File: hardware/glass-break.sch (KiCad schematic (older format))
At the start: 33 parts, among them P1 USB_OTG, SW1 SW_PUSH, SW2 SW_PUSH, SW3 SW_PUSH, U1 ESP-WROOM-02, U11 SPX3819, U2 OP275, U3 electret_microphone

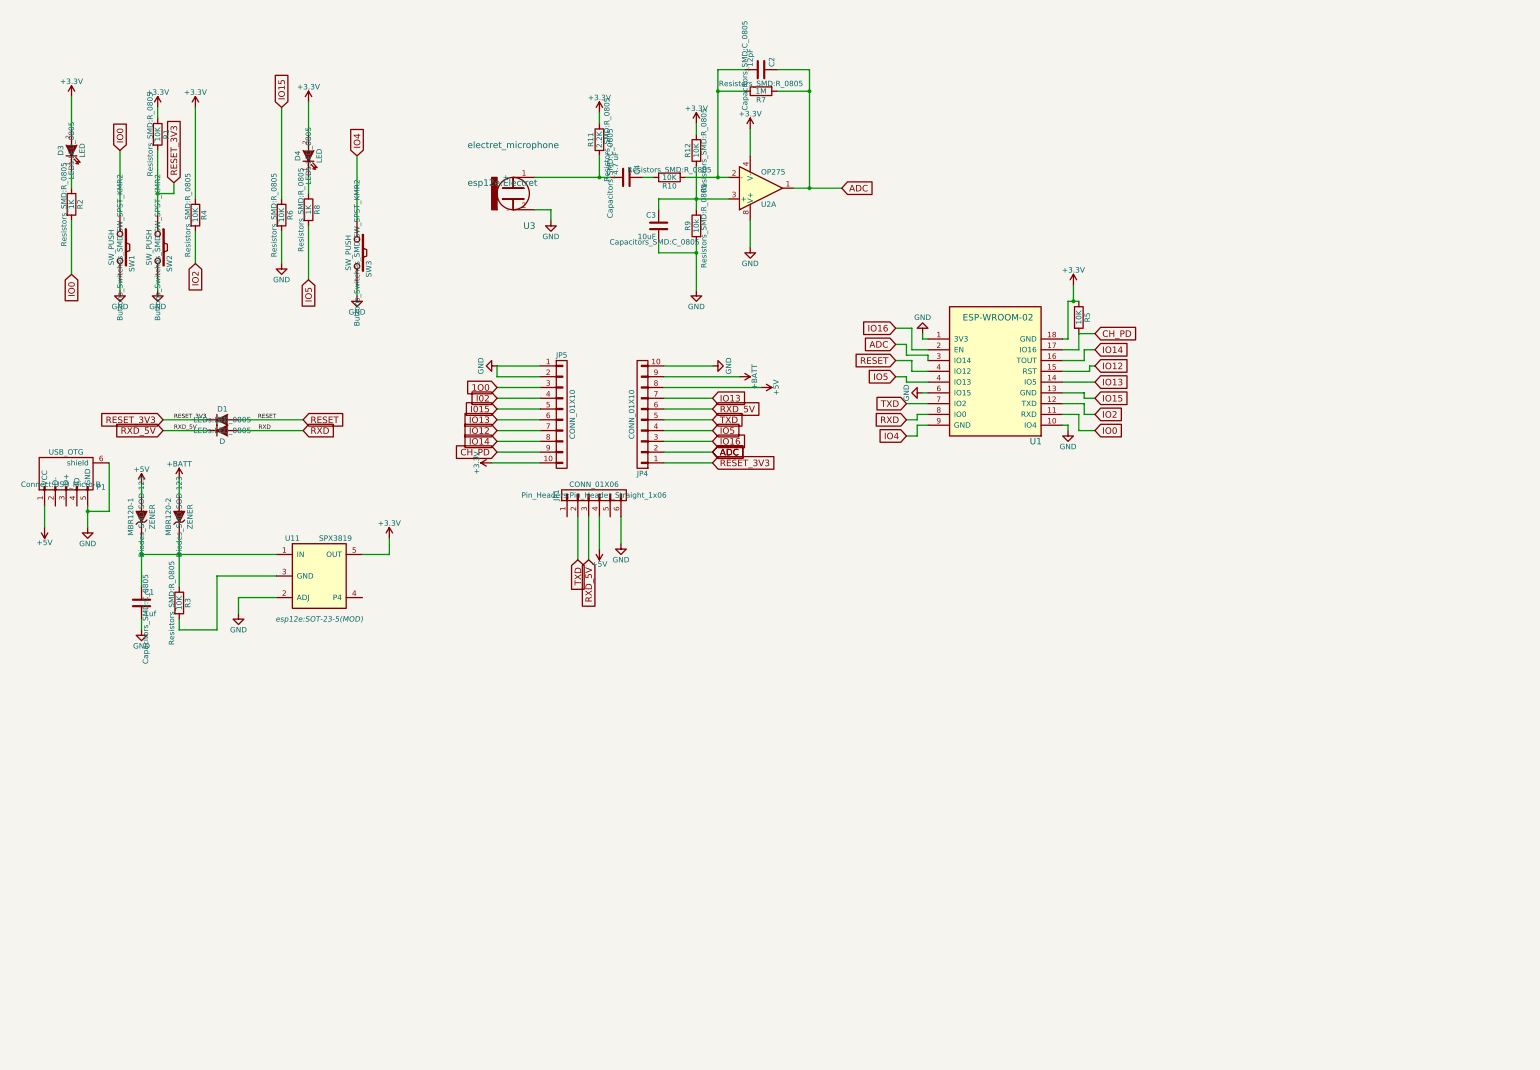
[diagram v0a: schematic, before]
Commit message: update
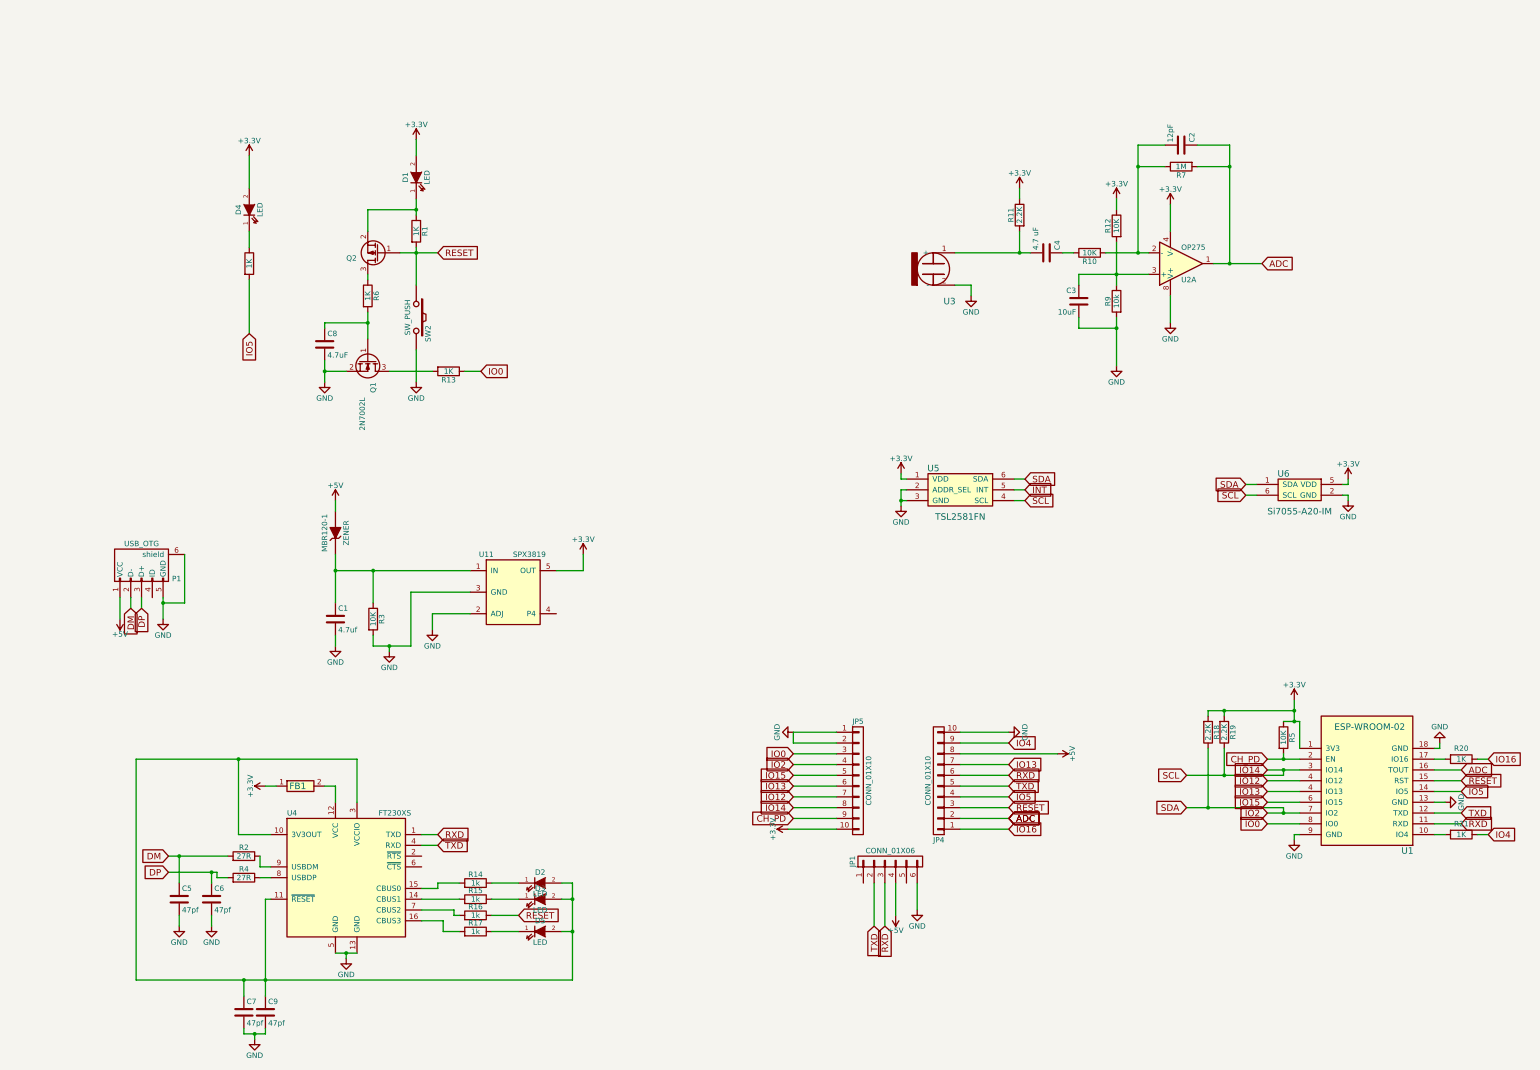
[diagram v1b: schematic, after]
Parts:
- removed D1, D2: D, LEDs:LED_0805, symbol D
- removed MBR120-2: ZENER, Diodes_SMD:SOD-123, symbol ZENER
- removed SW1, SW3: SW_PUSH, Buttons_Switches_SMD:SW_SPST_KMR2, symbol SW_PUSH
- added C5, C6, C7, C9: 47pf, Capacitors_SMD:C_0603, symbol C
- added C8: 4.7uF, Capacitors_SMD:C_0805, symbol C
- added D1, D2, D5: LED, LEDs:LED_0805, symbol LED
- added FB1: BLM18PG330SN1D, Resistors_SMD:R_0603, symbol BK0603HS330-T
- added Q1: 2N7002L, TO_SOT_Packages_SMD:SOT-23, symbol Q_NMOS_GSD
- added Q2: BSS84LT1G, TO_SOT_Packages_SMD:SOT-23, symbol Q_PMOS_GSD
- added R13, R20, R21: 1K, Resistors_SMD:R_0603, symbol R
- added R14, R15, R16, R17: 1k, Resistors_SMD:R_0603, symbol R
- added R18, R19: 2.2K, Resistors_SMD:R_0603, symbol R
- added U4: FT230XS, Housings_SSOP:SSOP-16_3.9x4.9mm_Pitch0.635mm, symbol FT230XS
- added U5: TSL2581FN, Housings_DFN_QFN:DFN-6-1EP_2x2mm_Pitch0.65mm, symbol TSL2581FN
- added U6: Si7055-A20-IM, Housings_DFN_QFN:DFN-6-1EP_3x3mm_Pitch0.95mm, symbol Si7055-A20-IM
- C1: value 1uf -> 4.7uf; Part Number (none) -> VJ0805G475KXYTW1BC
- C2: footprint Capacitors_SMD:C_0805 -> Resistors_SMD:R_0603
- C3: footprint Capacitors_SMD:C_0805 -> Capacitors_SMD:C_0603
- D4: Part Number (none) -> LS Q976-NR-1
- MBR120-1: Part Number (none) -> MBR120VLSFT1G
- P1: Part Number (none) -> 10118194-0001LF
- R1, R6: value 10K -> 1K; footprint Resistors_SMD:R_0805 -> Resistors_SMD:R_0603; Part Number (none) -> ERJ-3EKF1001V
- R10, R11, R12, R5, R7, R9: footprint Resistors_SMD:R_0805 -> Resistors_SMD:R_0603
- R2: value 1K -> 27R; footprint Resistors_SMD:R_0805 -> Resistors_SMD:R_0603
- R3: footprint Resistors_SMD:R_0805 -> Resistors_SMD:R_0603; Part Number (none) -> ERJ-3GEYJ103V
- R4: value 10K -> 27R; footprint Resistors_SMD:R_0805 -> Resistors_SMD:R_0603
- R8: footprint Resistors_SMD:R_0805 -> Resistors_SMD:R_0603; Part Number (none) -> ERJ-3EKF1001V
- SW2: Part Number (none) -> KMR211NG LFS
- U11: footprint esp12e:SOT-23-5(MOD) -> TO_SOT_Packages_SMD:SOT-23-5; Part Number (none) -> ERJ-3GEYJ103V
- U3: value electret_microphone -> CMC-5044PF-A
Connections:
- net +BATT is gone; now on net IO4: JP4.9 (P9)
- net 1O0 is gone; now on net IO0: JP5.3 (P3)
- net I015 is gone; now on net IO15: JP5.5 (P5)
- net I02 is gone; now on net IO2: JP5.4 (P4)
- net RXD_5V is gone; now on net RXD: JP1.3 (P3), JP4.6 (P6)
- net +3V3: now also U1.1 (3V3), D1.2 (A), FB1.1, R18.2, R19.2, U5.1 (VDD), U6.5 (VDD); no longer D3.2 (A), R1.1, R4.1, U1.18 (GND)
- net ADC: now also U1.16 (TOUT); no longer U1.3 (IO14)
- net CH_PD: now also U1.2 (EN); no longer U1.17 (IO16)
- net GND: now also R3.2, U1.13 (GND), U1.18 (GND), U1.9 (GND), U11.3 (GND), C5.2, C6.2, C7.2, C8.2, C9.2, Q1.2 (S), U4.13 (GND), U4.5 (GND), U5.2 (ADDR_SEL), U5.3 (GND), U6.2 (GND); no longer R6.2, U1.1 (3V3), U1.10 (IO4), U1.6 (IO15)
- net IO0: now also U1.8 (IO0), R13.1; no longer R2.2, U1.11 (RXD)
- net IO12: now also U1.4 (IO13); no longer U1.15 (RST)
- net IO13: now also U1.4 (IO13); no longer U1.14 (IO5)
- net IO14: now also U1.3 (IO14), R19.1, U5.4 (SCL), U6.6 (SCL); no longer U1.16 (TOUT)
- net IO15: now also U1.6 (IO15); no longer R6.1, U1.13 (GND)
- net IO16: now also JP4.1 (P1), R20.1; no longer JP4.3 (P3), U1.2 (EN)
- net IO2: now also U1.7 (IO2), R18.1, U5.6 (SDA), U6.1 (SDA); no longer R4.2, U1.12 (TXD)
- net IO4: now also R21.1; no longer U1.9 (GND)
- net IO5: now also U1.14 (IO5); no longer U1.4 (IO13)
- net RESET: now also JP4.3 (P3), R1.2, SW2.1, U1.15 (RST), Q2.1 (G), R16.1; no longer U1.4 (IO13)
- net RXD: now also U1.11 (RXD), U4.1 (TXD); no longer U1.8 (IO0)
- net TXD: now also U1.12 (TXD), U4.4 (RXD); no longer U1.7 (IO2)
- net DM: now reaches P1.2 (D-)
- net DM: now also R2.2, C5.1
- net DP: now reaches P1.3 (D+)
- net DP: now also R4.2, C6.1
- net at R2.1: now also U4.9 (USBDM); no longer D3.1 (K)
- removed net RESET_3V3: JP4.1 (P1), R1.2, SW2.1
- new net: D1.1 (K), Q2.2 (S), R1.1
- new net: R21.2, U1.10 (IO4)
- new net: R20.2, U1.17 (IO16)
- new net: FB1.2, U4.12 (VCC)
- new net: C7.1, C9.1, D2.2 (A), D3.2 (A), D5.2 (A), U4.10 (3V3OUT), U4.11 (~RESET), U4.3 (VCCIO)
- new net: R15.2, U4.14 (CBUS1)
- new net: R14.2, U4.15 (CBUS0)
- new net: R17.2, U4.16 (CBUS3)
- new net: R16.2, U4.7 (CBUS2)
- new net: R4.1, U4.8 (USBDP)
- new net: Q2.3 (D), R6.1
- new net: C8.1, Q1.1 (G), R6.2
- new net: Q1.3 (D), R13.2
- new net: D2.1 (K), R14.1
- new net: D3.1 (K), R15.1
- new net: D5.1 (K), R17.1
- new net INT: U5.5 (INT)
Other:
- moved on the sheet: C1, C2, C3, C4, D4, JP1, JP4, JP5, MBR120-1, P1, R1, R10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
